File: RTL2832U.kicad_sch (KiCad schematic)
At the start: 40 parts, among them U5 RTL2832U, U6 M24C02-WMN

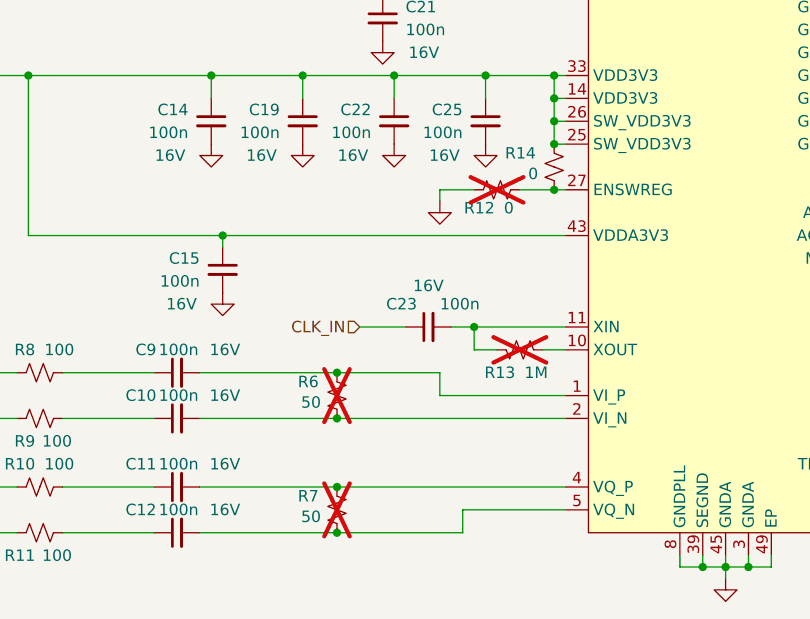
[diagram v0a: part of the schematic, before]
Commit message: Small PCB layout tweaks
Beautification, if you will...
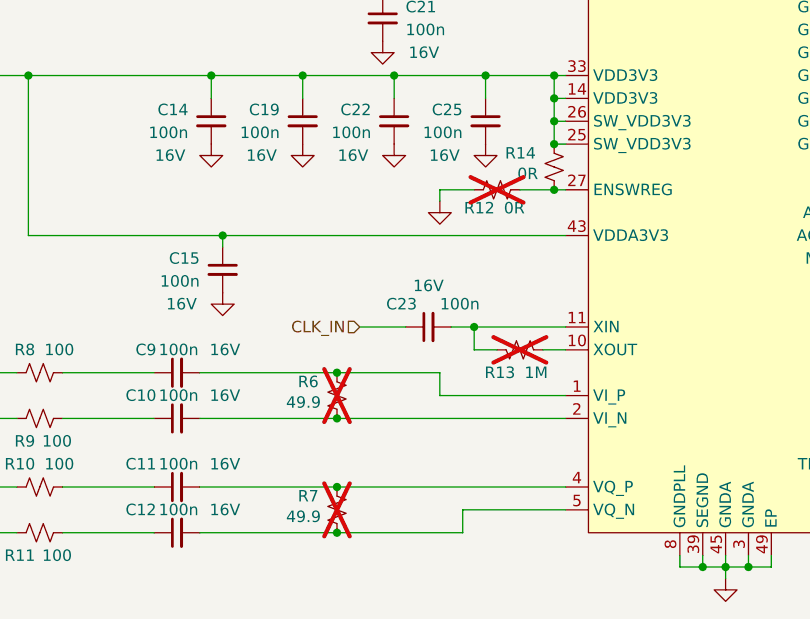
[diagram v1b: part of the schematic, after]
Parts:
- R12, R14: value 0 -> 0R
- R6, R7: value 50 -> 49.9
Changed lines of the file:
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@@
 			)
 		)
-		(property "Value" "0"
+		(property "Value" "0R"
 			(at 162.052 164.592 90)
 			(show_name no)
@@
 			)
 		)
-		(property "Value" "50"
+		(property "Value" "49.9"
 			(at 141.732 186.182 0)
 			(show_name no)
@@
 			)
 		)
-		(property "Value" "0"
+		(property "Value" "0R"
 			(at 165.862 160.782 0)
 			(show_name no)
@@
 			)
 		)
-		(property "Value" "50"
+		(property "Value" "49.9"
 			(at 141.732 198.882 0)
 			(show_name no)
